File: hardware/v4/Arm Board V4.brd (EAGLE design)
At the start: 108 x 50.8 mm, 38 parts, among them IC3 L6206D, P1 STELLARIS-LAUNCHPADSTELLARIS-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, U1 SN74LS241DW, U2 XBEE-1B3

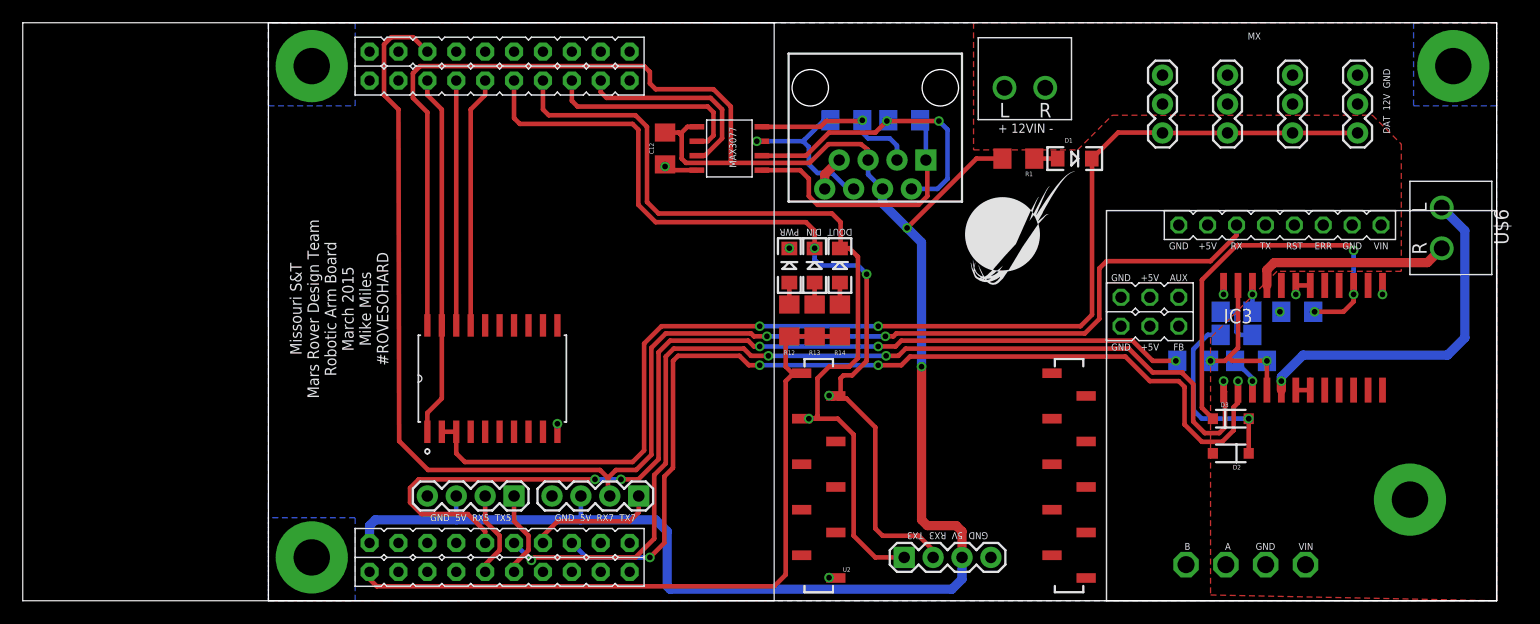
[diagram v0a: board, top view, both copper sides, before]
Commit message: cleaned up robo arm a bit
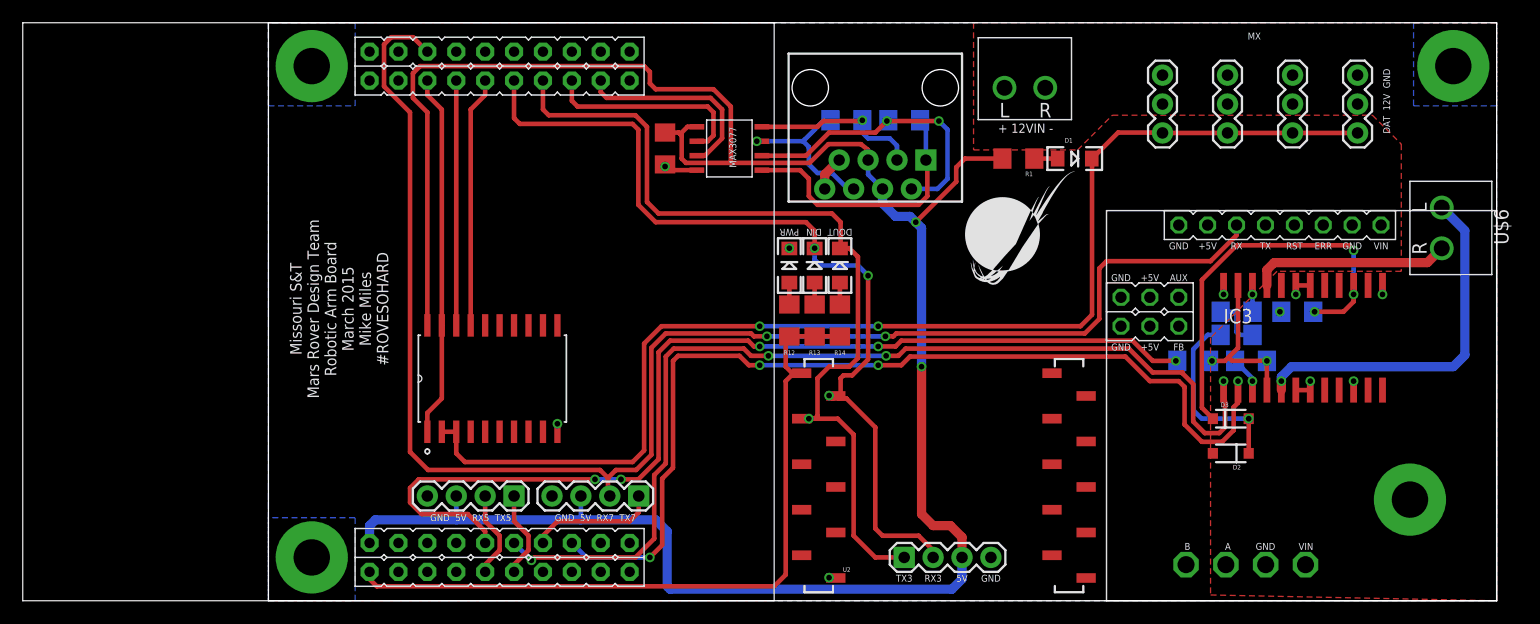
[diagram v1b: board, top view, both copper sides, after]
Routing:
- net A1: track 31.0 -> 31.9 mm
- net GND: track 16.8 -> 17.6 mm, vias 8 -> 10
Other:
- board text added: "5V"
- board text added: "GND"
- board text added: "RX3"
- board text added: "TX3"
- board text removed: "GND 5V RX3 TX3"
